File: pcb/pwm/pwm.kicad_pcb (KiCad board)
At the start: 2 copper layers, 154.9 x 152.4 mm, 12 parts, among them Q1 IRFB4321PBF, Q2 IRFB4321PBF, Q3 IRFB4321PBF, Q4 IRFB4321PBF, Q5 IRFB4321PBF, Q6 IRFB4321PBF, Q7 IRFB4321PBF, Q8 IRFB4321PBF

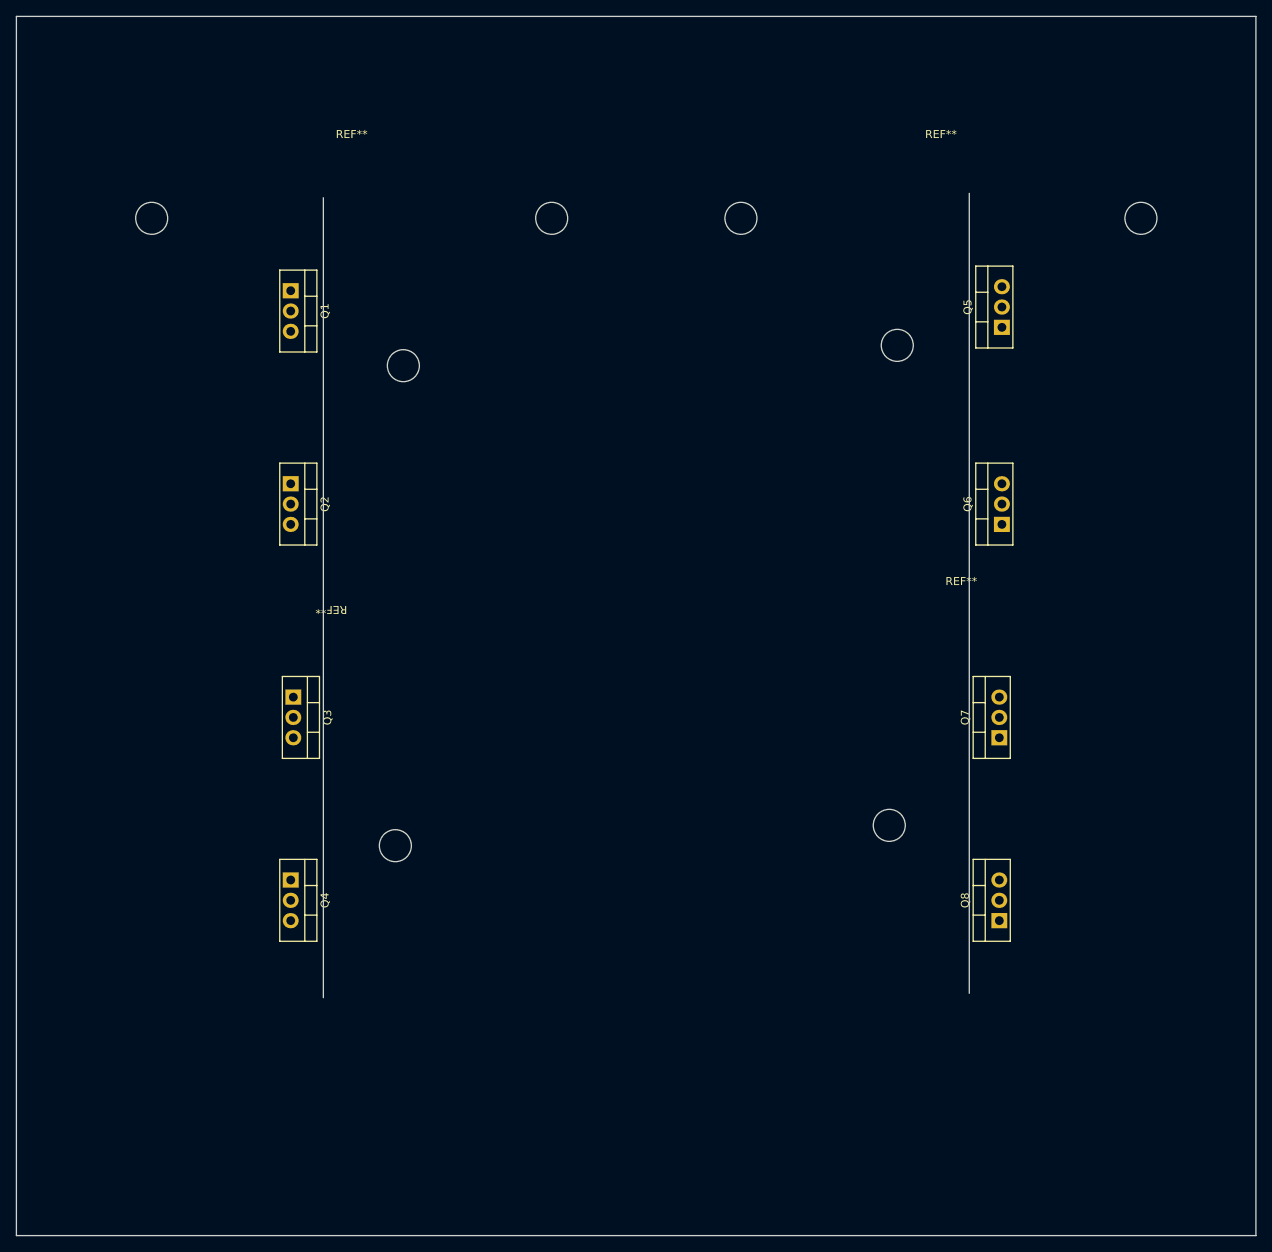
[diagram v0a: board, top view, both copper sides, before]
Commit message: Signed-off-by: Dmitry Ponyatov <dponyatov@samsa.local>
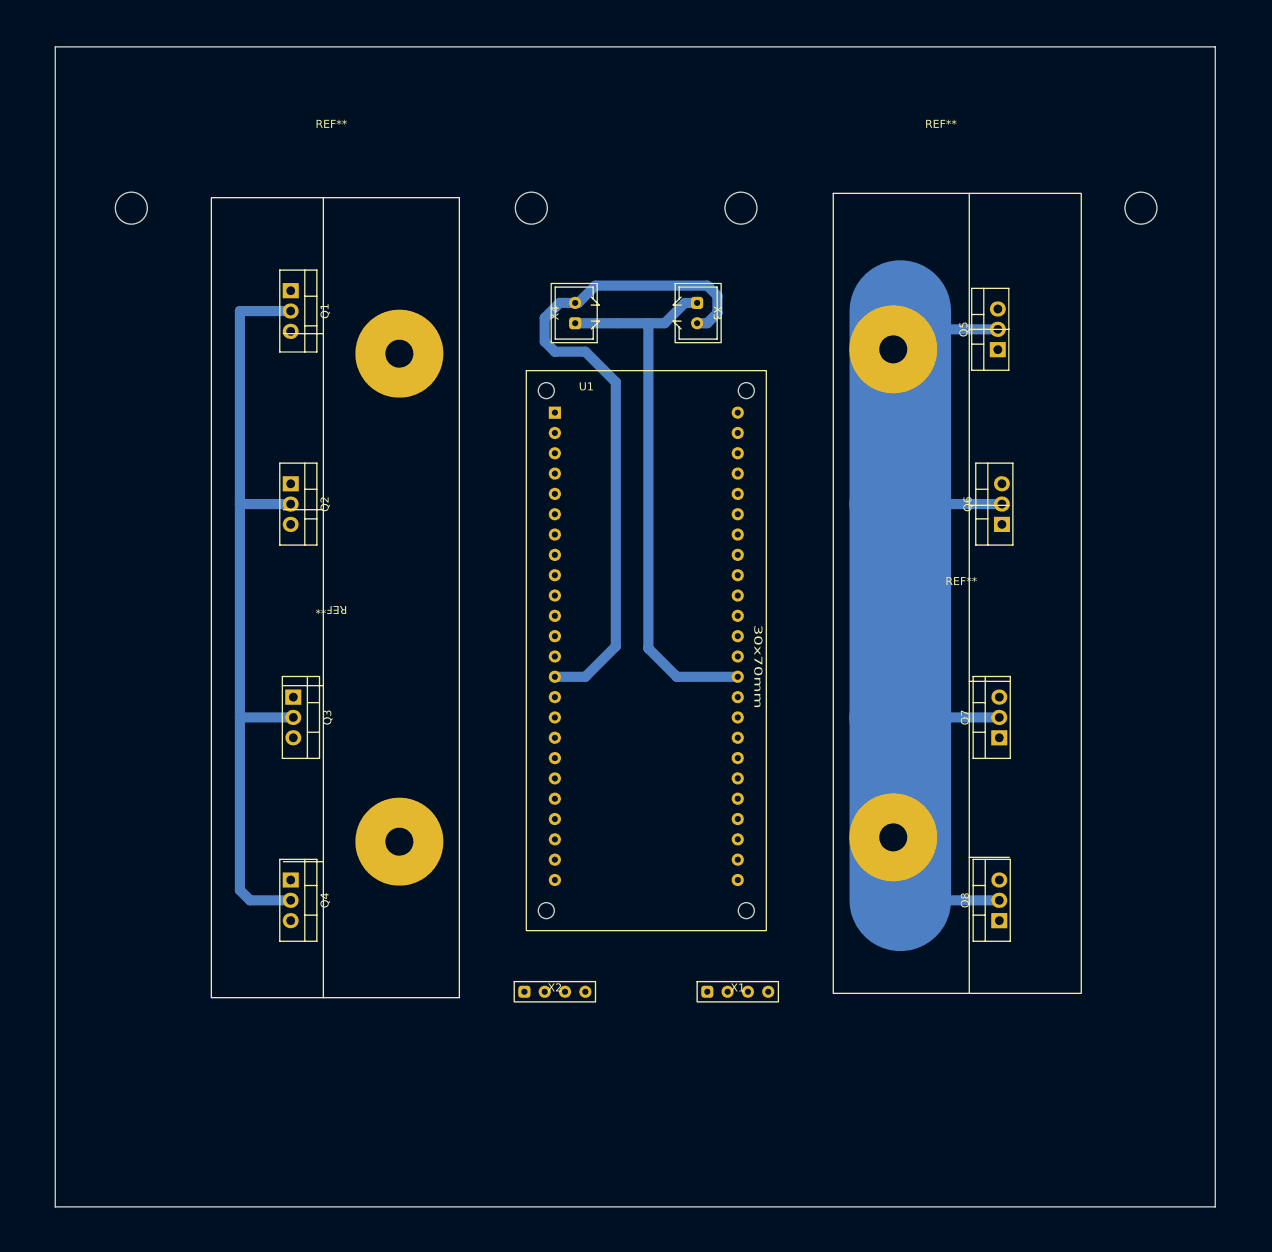
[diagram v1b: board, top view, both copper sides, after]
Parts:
- added U1: pwm_meson0, pwm_meson:pwm_meson0, F.Cu at (95.2, 106.7)
- added X1: Conn_01x04_Male, terminal:PLS-4, F.Cu at (106.7, 147.3)
- added X2: Conn_01x04_Male, terminal:PLS-4, F.Cu at (83.8, 147.3)
- added X3: Conn_01x02_Male, terminal:CWF-2, F.Cu at (101.6, 62.5)
- added X4: Fan, terminal:CWF-2, F.Cu at (86.4, 62.5)
- moved REF** 2.84 mm to (55.9, 39.4)
- moved Q5 2.83 mm to (139.2, 67.1)
- moved REF** 1.27 mm to (132.1, 39.4)
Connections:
- net Net-(Q5-Pad1) renamed /G5
- net Net-(Q6-Pad1) renamed /G6
- net Net-(Q7-Pad1) renamed /G7
- net Net-(Q8-Pad1) renamed /G8
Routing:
- net /phase: track 0.00 -> 123.1 mm
- net /+60V: track 0.00 -> 98.6 mm
- net /fan+: track 0.00 -> 85.2 mm
- net /fan-: track 0.00 -> 69.6 mm
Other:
- board size 154.9 x 152.4 mm -> 145 x 145 mm
